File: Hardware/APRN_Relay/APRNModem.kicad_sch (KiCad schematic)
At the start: 7 parts, among them J201 Conn_Coaxial, U201 DRA818V

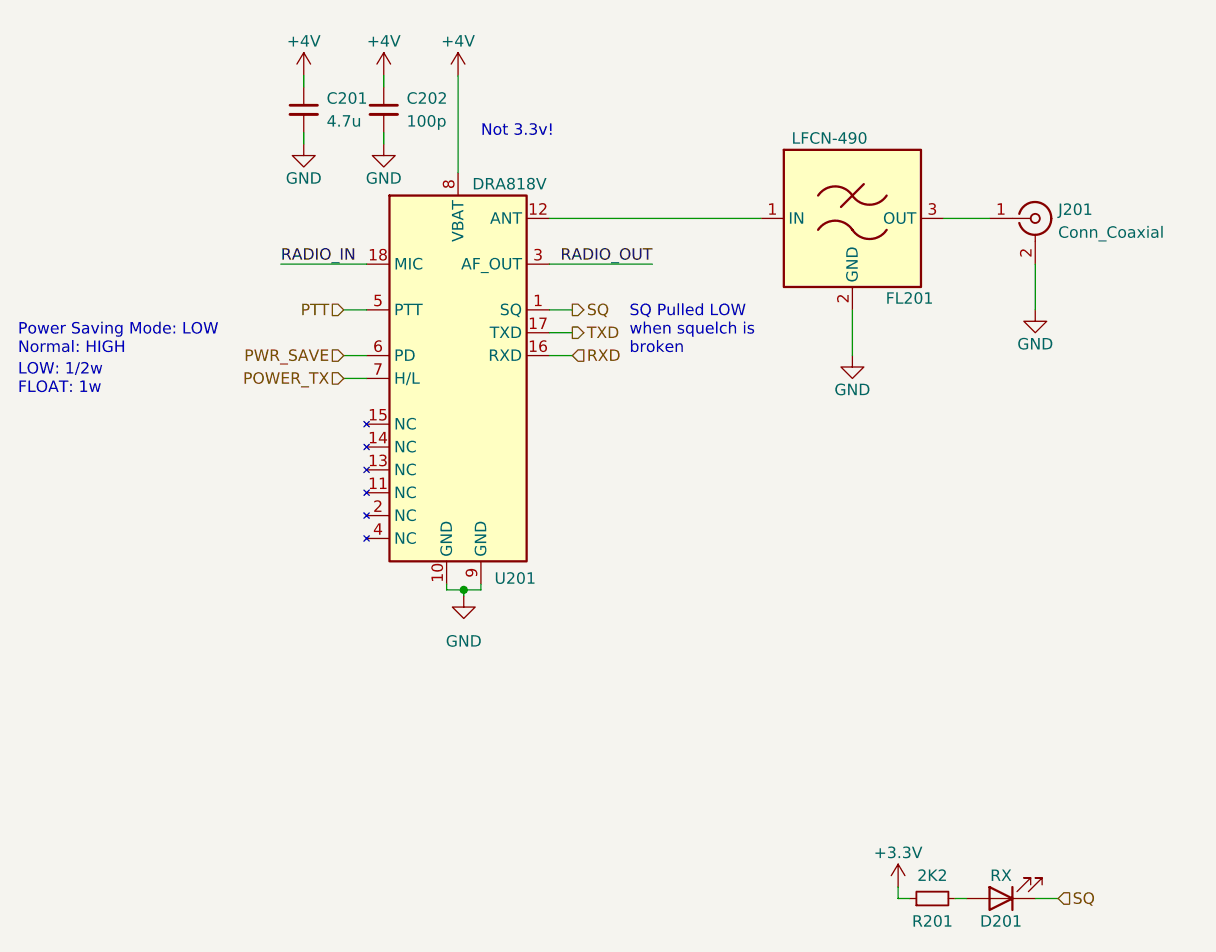
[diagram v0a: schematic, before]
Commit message: Even prettier
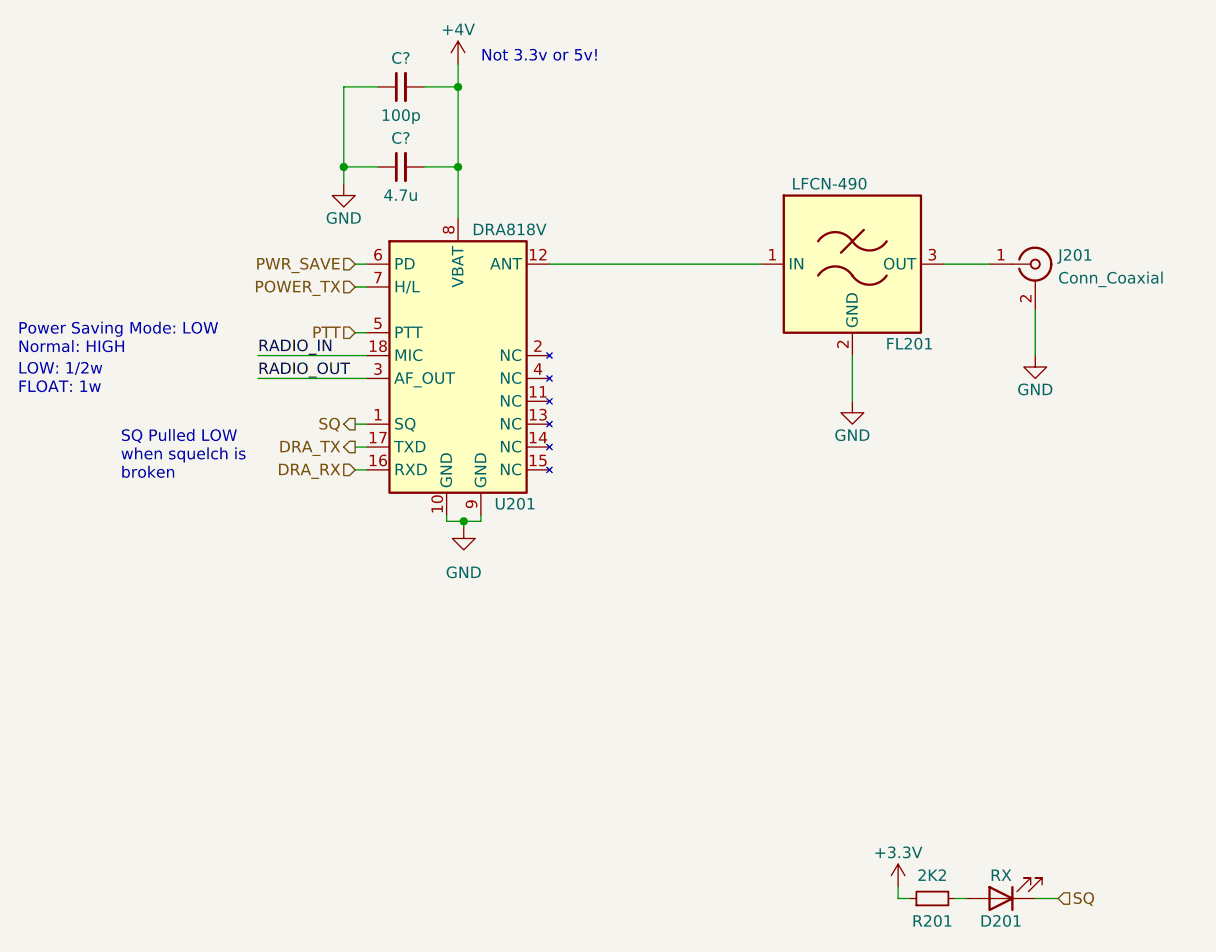
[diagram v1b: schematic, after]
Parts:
- removed C201: 4.7u, Capacitor_SMD:C_0805_2012Metric, symbol Device:C_Small
- removed C202: 100p, Capacitor_SMD:C_0805_2012Metric, symbol Device:C_Small
- added C?: 100p, Capacitor_SMD:C_0805_2012Metric, symbol Device:C_Small
- added C?: 4.7u, Capacitor_SMD:C_0805_2012Metric, symbol Device:C_Small
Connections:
- net +4V: now also C?.2, C?.2
- net GND: now also C?.1, C?.1
- net RXD renamed DRA_RX
- net TXD renamed DRA_TX
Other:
- note added: "Not 3.3v or 5v!"
- note removed: "Not 3.3v!"
- moved on the sheet: FL201, J201, U201
